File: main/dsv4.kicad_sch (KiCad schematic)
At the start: 2 parts, among them J101 Conn_01x02, J102 Conn_01x02

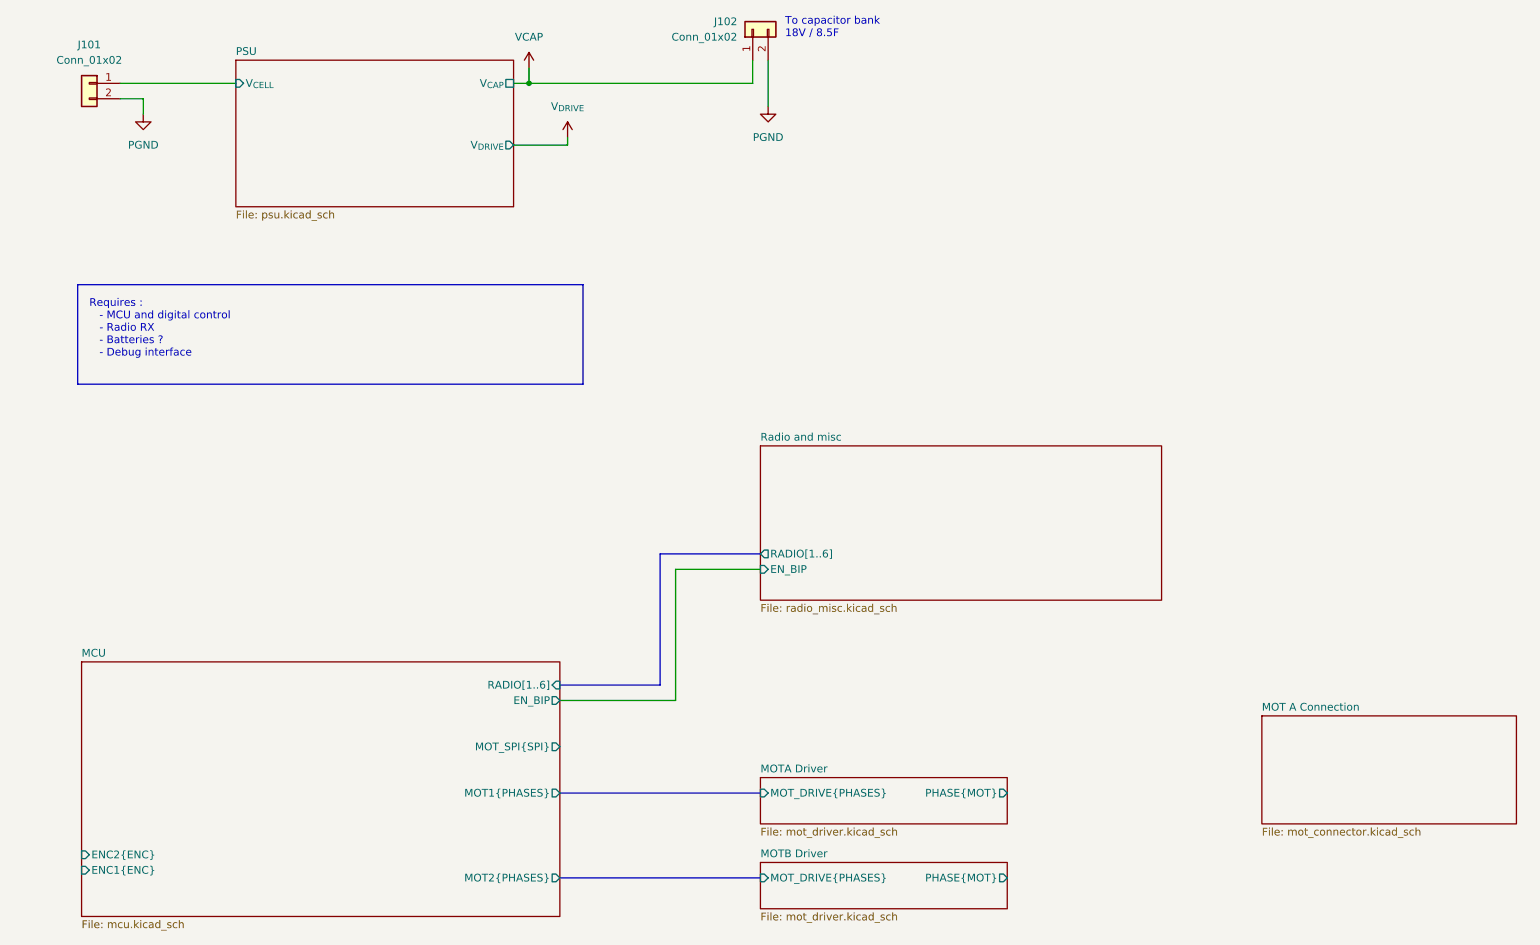
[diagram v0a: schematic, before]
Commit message: Update, with FTDI, mostly OK
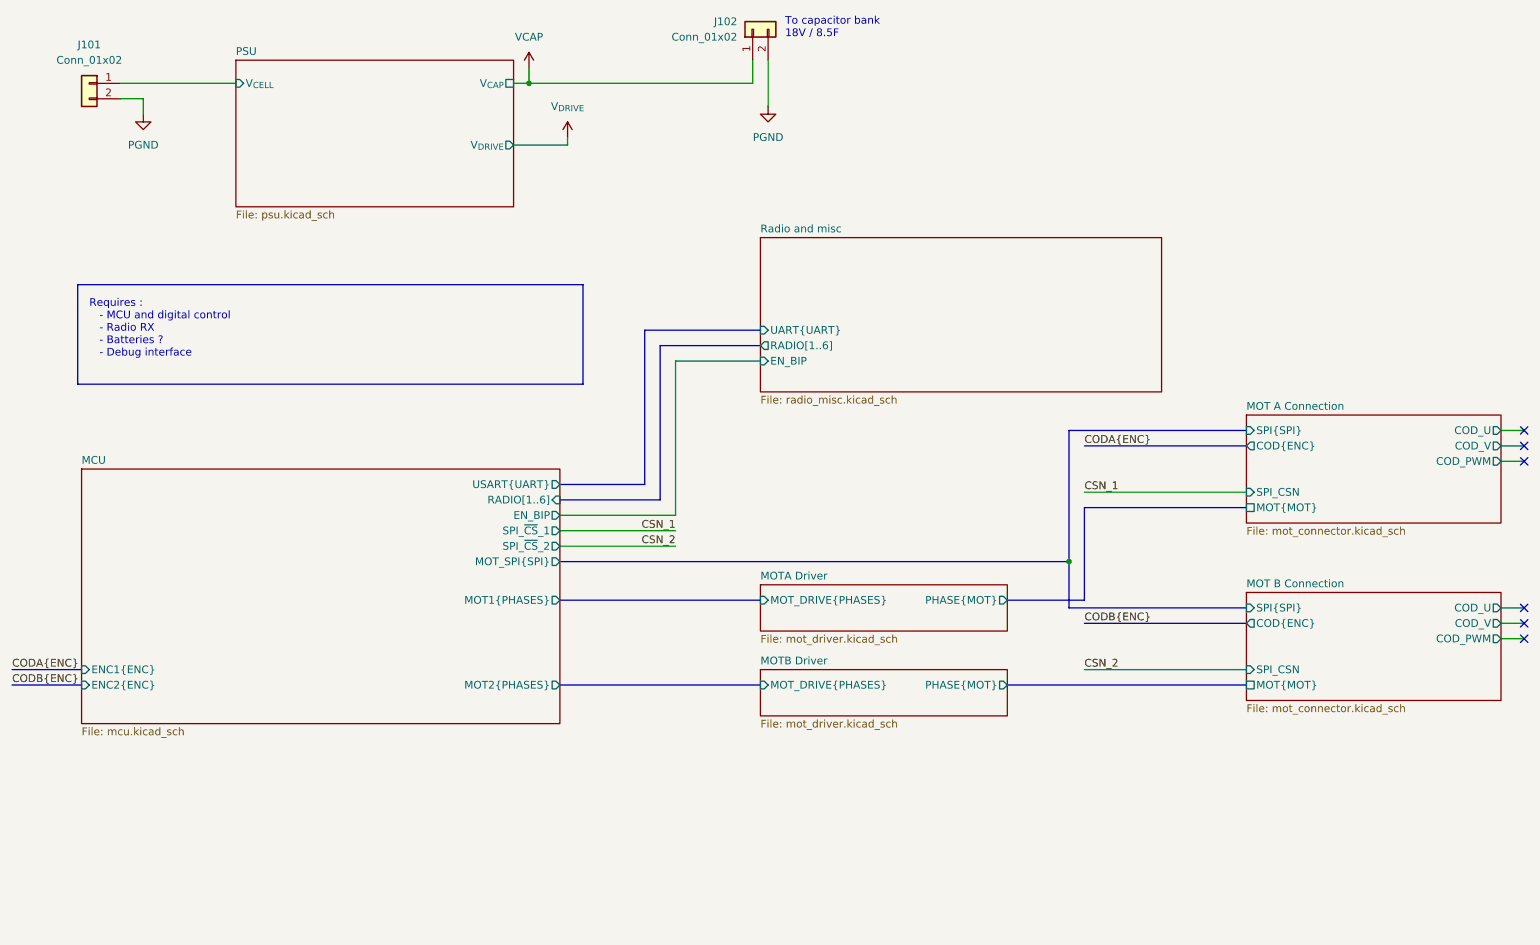
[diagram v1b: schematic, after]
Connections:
- no-connect marks 0 -> 6
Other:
- added sheet MOT B Connection (mot_connector.kicad_sch)
- sheet MCU ports: added SPI_~{CS}_1, SPI_~{CS}_2, USART{UART}; removed none
- sheet MOT A Connection ports: added COD_PWM, COD_U, COD_V, COD{ENC}, MOT{MOT}, SPI_CSN, SPI{SPI}; removed none
- sheet Radio and misc ports: added UART{UART}; removed none
